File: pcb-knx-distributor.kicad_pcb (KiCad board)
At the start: 2 copper layers, 113.5 x 28 mm, 21 parts, among them J1 Conn_01x02_Pin, J10 Conn_01x02_Pin, J11 Conn_01x02_Pin, J12 Conn_01x02_Pin, J13 Conn_01x02_Pin, J14 Conn_01x02_Pin, J2 Conn_01x02_Pin, J3 Conn_01x02_Pin, J4 Conn_01x02_Pin, J5 Conn_01x02_Pin, J6 Conn_01x02_Pin, J7 Conn_01x02_Pin, J8 Conn_01x02_Pin, J9 Conn_01x02_Pin

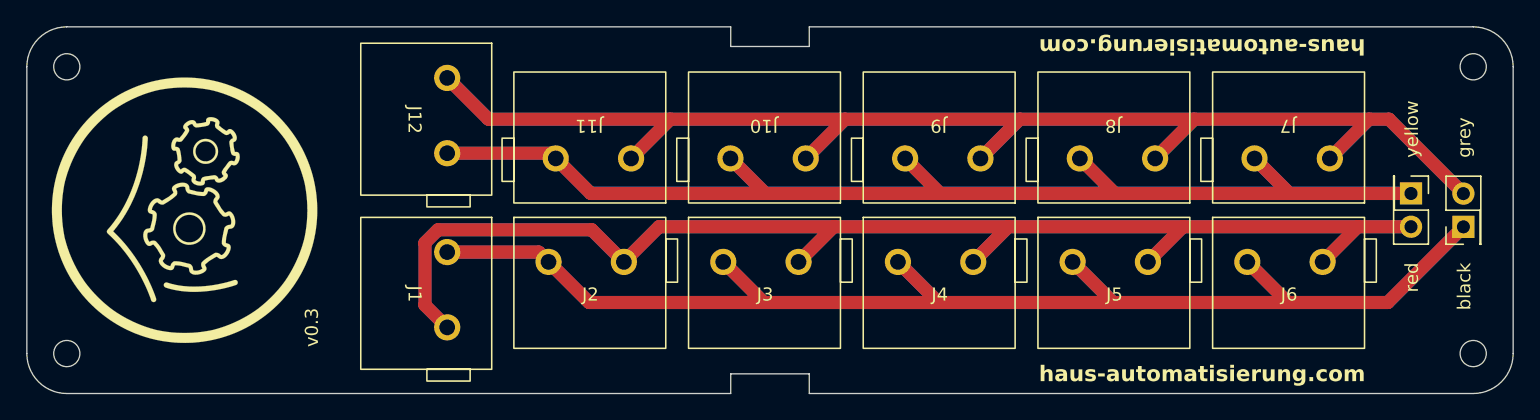
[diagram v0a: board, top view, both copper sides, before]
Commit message: 0.4
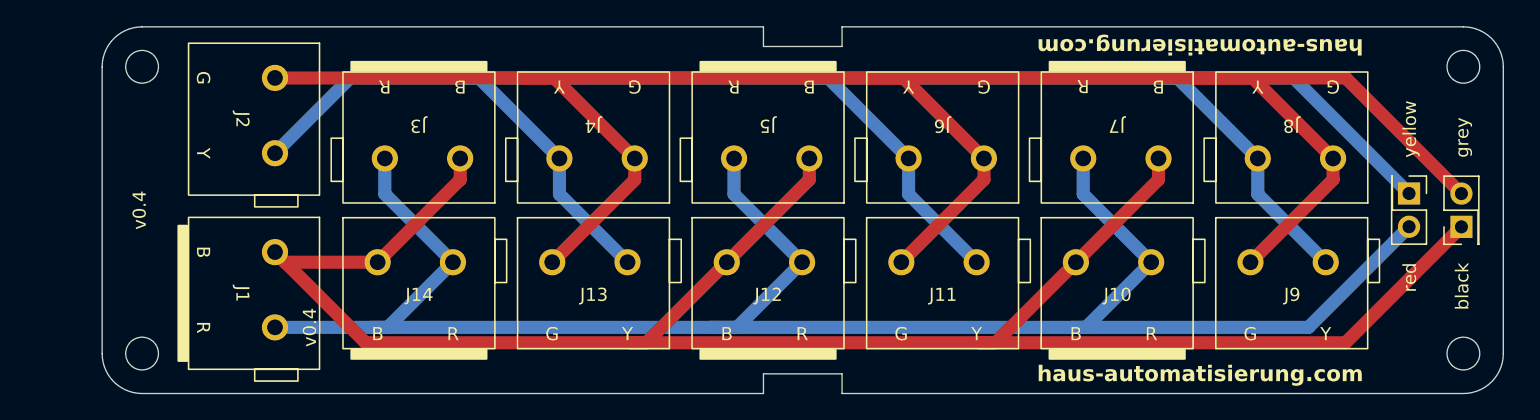
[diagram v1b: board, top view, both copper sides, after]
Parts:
- removed G***: LOGO, haus-automatisierung:Logo_20mm
- removed G***: LOGO, haus-automatisierung:QRCode-hausauto_20mm
- removed the REF** at (25.3, 53.0)
- removed the REF** at (132.7, 53.0)
- removed the REF** at (132.7, 75.0)
- removed the REF** at (25.3, 75.0)
- added J14: Conn_01x02_Pin, haus-automatisierung:Wago-243-211, F.Cu at (46.4, 64.6)
- added J8: Conn_01x02_Pin, haus-automatisierung:Wago-243-212, F.Cu at (124.7, 63.5)
- added REF**: MountingHole_2.5mm, MountingHole:MountingHole_2.5mm, F.Cu at (131.9, 53.0)
- added REF**: MountingHole_2.5mm, MountingHole:MountingHole_2.5mm, F.Cu at (31.1, 53.0)
- added REF**: MountingHole_2.5mm, MountingHole:MountingHole_2.5mm, F.Cu at (131.9, 75.0)
- added REF**: MountingHole_2.5mm, MountingHole:MountingHole_2.5mm, F.Cu at (31.1, 75.0)
- added REF**: KiCad-Logo2_6mm_SilkScreen, Symbol:KiCad-Logo2_6mm_SilkScreen, B.Cu at (34.4, 64.0)
- J11: renamed from J4; footprint haus-automatisierung:Wago-243-211 -> haus-automatisierung:Wago-243-212
- J13: renamed from J2; footprint haus-automatisierung:Wago-243-211 -> haus-automatisierung:Wago-243-212
- J3: renamed from J11; footprint haus-automatisierung:Wago-243-212 -> haus-automatisierung:Wago-243-211
- J5: renamed from J9; footprint haus-automatisierung:Wago-243-212 -> haus-automatisierung:Wago-243-211
- J7: footprint haus-automatisierung:Wago-243-212 -> haus-automatisierung:Wago-243-211
- J9: renamed from J6; footprint haus-automatisierung:Wago-243-211 -> haus-automatisierung:Wago-243-212
- moved REF** 72.4 mm to (121.5, 64.0)
- moved J1 13.1 mm to (44.6, 64.5)
- moved J2 13.1 mm to (44.6, 51.2)
- moved J7 13.1 mm to (111.3, 63.5)
- moved J6 13.1 mm to (98.0, 63.5)
- moved J5 13.1 mm to (84.7, 63.5)
- moved J4 13.1 mm to (71.3, 63.5)
- moved J3 13.1 mm to (58.0, 63.5)
- moved J13 0.28 mm to (59.7, 64.6)
- moved J12 0.27 mm to (73.0, 64.6)
- moved J11 0.26 mm to (86.4, 64.6)
- moved J10 0.25 mm to (99.7, 64.6)
- moved J9 0.24 mm to (113.0, 64.6)
- moved J16 0.15 mm to (127.8, 62.7)
- moved J15 0.15 mm to (131.8, 65.3)
- renumbered J5 to J10, J3 to J12, J13 to J15, J14 to J16, J12 to J2, J10 to J4, J8 to J6
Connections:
- J11 pad 1: /black -> /grey
- J11 pad 2: /red -> /yellow
- J13 pad 1: /black -> /grey
- J13 pad 2: /red -> /yellow
- J3 pad 1: /grey -> /black
- J3 pad 2: /yellow -> /red
- J5 pad 1: /grey -> /black
- J5 pad 2: /yellow -> /red
- J7 pad 1: /grey -> /black
- J7 pad 2: /yellow -> /red
- J9 pad 1: /black -> /grey
- J9 pad 2: /red -> /yellow
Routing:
- net /red: track 200.4 -> 145.6 mm
- net /grey: track 205.0 -> 161.5 mm
- net /black: track 198.3 -> 156.8 mm
- net /yellow: track 180.0 -> 153.1 mm
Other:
- board size 113.5 x 28 mm -> 107 x 28 mm
- board text added: "B"
- board text added: "G"
- board text added: "R"
- board text added: "Y"
- board text added: "v0.4"
- board text removed: "v0.3"
